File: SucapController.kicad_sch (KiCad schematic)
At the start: 44 parts, among them J1 Conn_01x14, J2 Conn_01x04, J3 Conn_01x02, J4 Conn_02x03_Counter_Clockwise, J5 Conn_02x03_Counter_Clockwise, J6 Conn_02x03_Counter_Clockwise, J7 Screw_Terminal_01x01, Q1 SI2301, U1 HX9193, U2 HX9193, U3 W25Q32JVSS, U4 STM32H750VBTx, U5 REF3030, U6 74LVC1G17, Y1 25M, Y2 32.768K

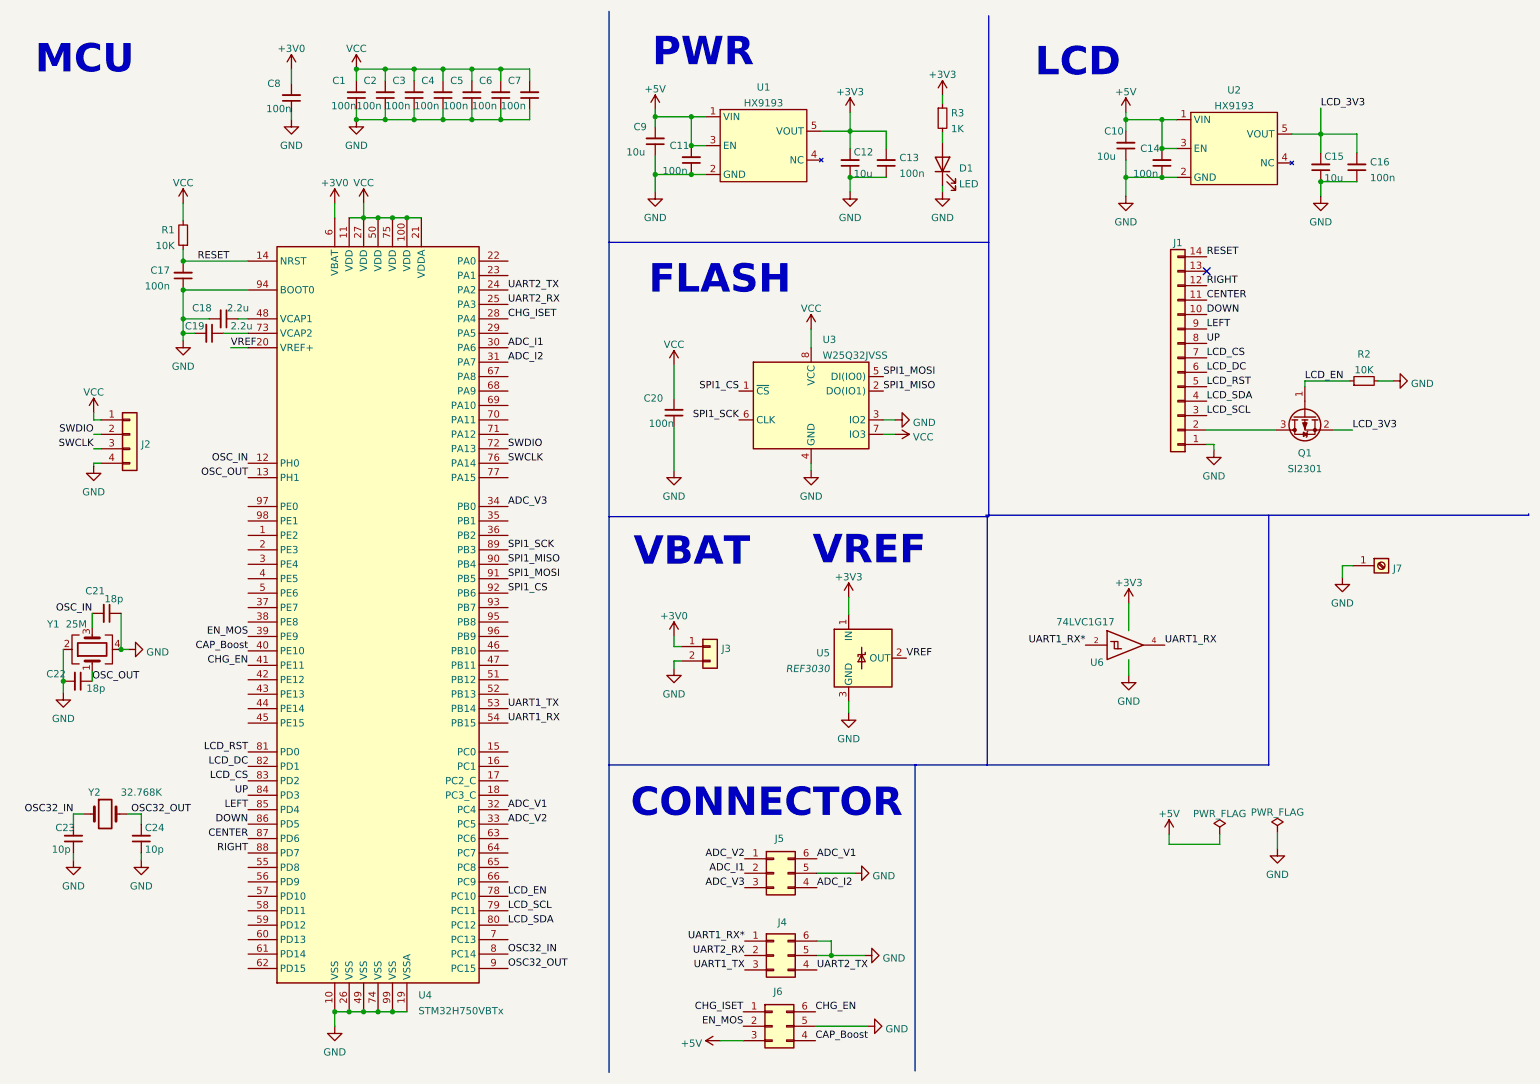
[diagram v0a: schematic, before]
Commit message: Do some change
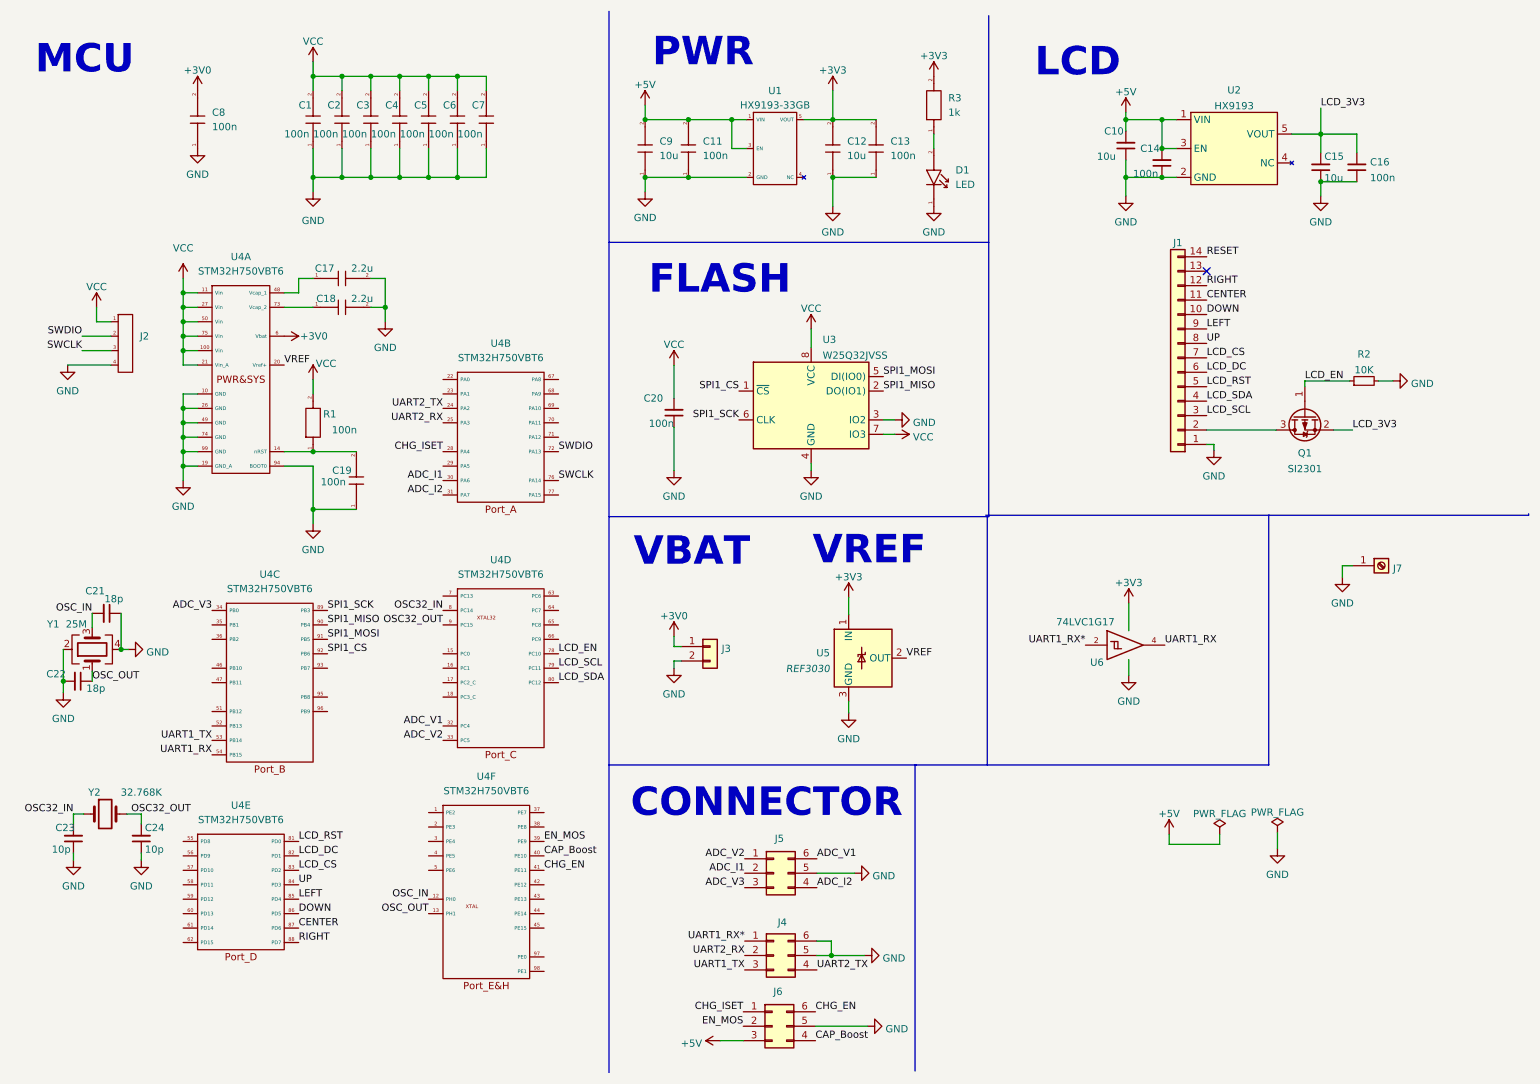
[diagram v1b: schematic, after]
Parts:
- removed C1, C11, C13, C17, C2, C3, C4, C5, C6, C7, C8: 100n, Capacitor_SMD:C_0603_1608Metric, symbol Device:C_Small
- removed C12, C9: 10u, Capacitor_SMD:C_0603_1608Metric, symbol Device:C_Small
- removed C18, C19: 2.2u, Capacitor_SMD:C_0603_1608Metric, symbol Device:C_Small
- removed D1: LED, LED_SMD:LED_0603_1608Metric, symbol Device:LED
- removed J2: Conn_01x04, Connector_JST:JST_GH_SM04B-GHS-TB_1x04-1MP_P1.25mm_Horizontal, symbol Connector_Generic:Conn_01x04
- removed R1: 10K, Resistor_SMD:R_0603_1608Metric, symbol Device:R_Small
- removed R3: 1K, Resistor_SMD:R_0603_1608Metric, symbol Device:R_Small
- removed U1: HX9193, Package_TO_SOT_SMD:SOT-23-5_HandSoldering, symbol MyLib:HX9193
- removed U4: STM32H750VBTx, Package_QFP:LQFP-100_14x14mm_P0.5mm, symbol MCU_ST_STM32H7:STM32H750VBTx
- added C1, C11, C13, C19, C2, C3, C4, C5, C6, C7, C8: 100n, GENERAL_RCL_SMD:C0603(1608M), symbol Basic_passive_components:Capacitor
- added C12, C9: 10u, GENERAL_RCL_SMD:C0603(1608M), symbol Basic_passive_components:Capacitor
- added C17, C18: 2.2u, GENERAL_RCL_SMD:C0603(1608M), symbol Basic_passive_components:Capacitor
- added D1: LED, symbol Basic_semiconductor:Diode_LED
- added J2: (no value), symbol Link_W2B_connector:Conn_01x04
- added R1: 100n, GENERAL_RCL_SMD:R0603(1608M), symbol Basic_passive_components:Resistor
- added R3: 1k, GENERAL_RCL_SMD:R0603(1608M), symbol Basic_passive_components:Resistor
- added U1: HX9193-33GB, GENERAL_SMALL-SEMI_SMD:SOT-23-5, symbol Power_LDO:HX9193-33GB
- added U4: STM32H750VBT6, GENERAL_LARGE-SEMI_SMD:QFP-1414_100, symbol Integrated-circuit_micro-controller:STM32H750VBT6
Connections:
- net +3V0: now also C8.2, U4.6 (Vbat)
- net +3V3: now also C1.2, C12.2, C13.2, C2.2, C3.2, C4.2, C5.2, C6.2, C7.2, J2.1, R1.2, R3.2, U1.5 (VOUT), U4.100 (Vin), U4.11 (Vin), U4.21 (Vin_A), U4.27 (Vin), U4.50 (Vin), U4.75 (Vin)
- net +5V: now also C11.2, C9.2, U1.1 (VIN), U1.3 (EN)
- net ADC_I1: now also U4.30 (PA6)
- net ADC_I2: now also U4.31 (PA7)
- net ADC_V1: now also U4.32 (PC4)
- net ADC_V2: now also U4.33 (PC5)
- net ADC_V3: now also U4.34 (PB0)
- net CAP_Boost: now also U4.40 (PE10)
- net CENTER: now also U4.87 (PD6)
- net CHG_EN: now also U4.41 (PE11)
- net CHG_ISET: now also U4.28 (PA4)
- net DOWN: now also U4.86 (PD5)
- net EN_MOS: now also U4.39 (PE9)
- net GND: now also C1.1, C11.1, C12.1, C13.1, C17.2, C18.2, C19.1, C2.1, C3.1, C4.1, C5.1, C6.1, C7.1, C8.1, C9.1, D1.1 (Cathode), J2.4, U1.2 (GND), U4.10 (GND), U4.19 (GND_A), U4.26 (GND), U4.49 (GND), U4.74 (GND), U4.94 (BOOT0), U4.99 (GND)
- net LCD_CS: now also U4.83 (PD2)
- net LCD_DC: now also U4.82 (PD1)
- net LCD_EN: now also U4.78 (PC10)
- net LCD_RST: now also U4.81 (PD0)
- net LCD_SCL: now also U4.79 (PC11)
- net LCD_SDA: now also U4.80 (PC12)
- net LEFT: now also U4.85 (PD4)
- net OSC32_IN: now also U4.8 (PC14)
- net OSC32_OUT: now also U4.9 (PC15)
- net OSC_IN: now also U4.12 (PH0)
- net OSC_OUT: now also U4.13 (PH1)
- net RIGHT: now also U4.88 (PD7)
- net SPI1_CS: now also U4.92 (PB6)
- net SPI1_MISO: now also U4.90 (PB4)
- net SPI1_MOSI: now also U4.91 (PB5)
- net SPI1_SCK: now also U4.89 (PB3)
- net SWCLK: now also J2.3, U4.76 (PA14)
- net SWDIO: now also J2.2, U4.72 (PA13)
- net UART1_RX: now also U4.54 (PB15)
- net UART1_TX: now also U4.53 (PB14)
- net UART2_RX: now also U4.25 (PA3)
- net UART2_TX: now also U4.24 (PA2)
- net UP: now also U4.84 (PD3)
- net VREF: now also U4.20 (Vref+)
- new net: C19.2, R1.1, U4.14 (nRST)
- new net: C17.1, U4.48 (Vcap_1)
- new net: D1.2 (Anode), R3.1
- new net: C18.1, U4.73 (Vcap_2)
